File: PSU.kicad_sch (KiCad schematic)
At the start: 39 parts, among them Q401 2N7002, SW401 SW_Push, SW402 SW_Push, U3 TPPM0110DWPR, U402 AP7381-33SA-7, U403 AP63200WU

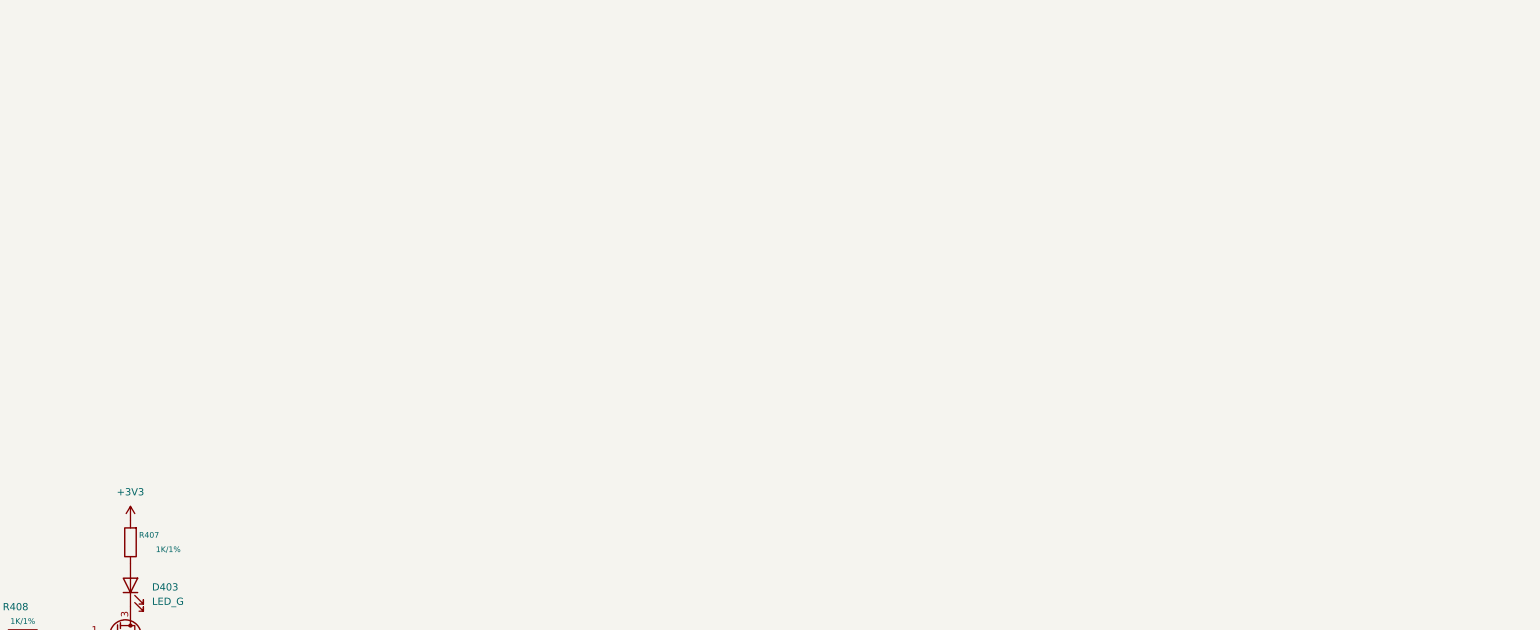
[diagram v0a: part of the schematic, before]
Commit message: some power stuff (unfinished)
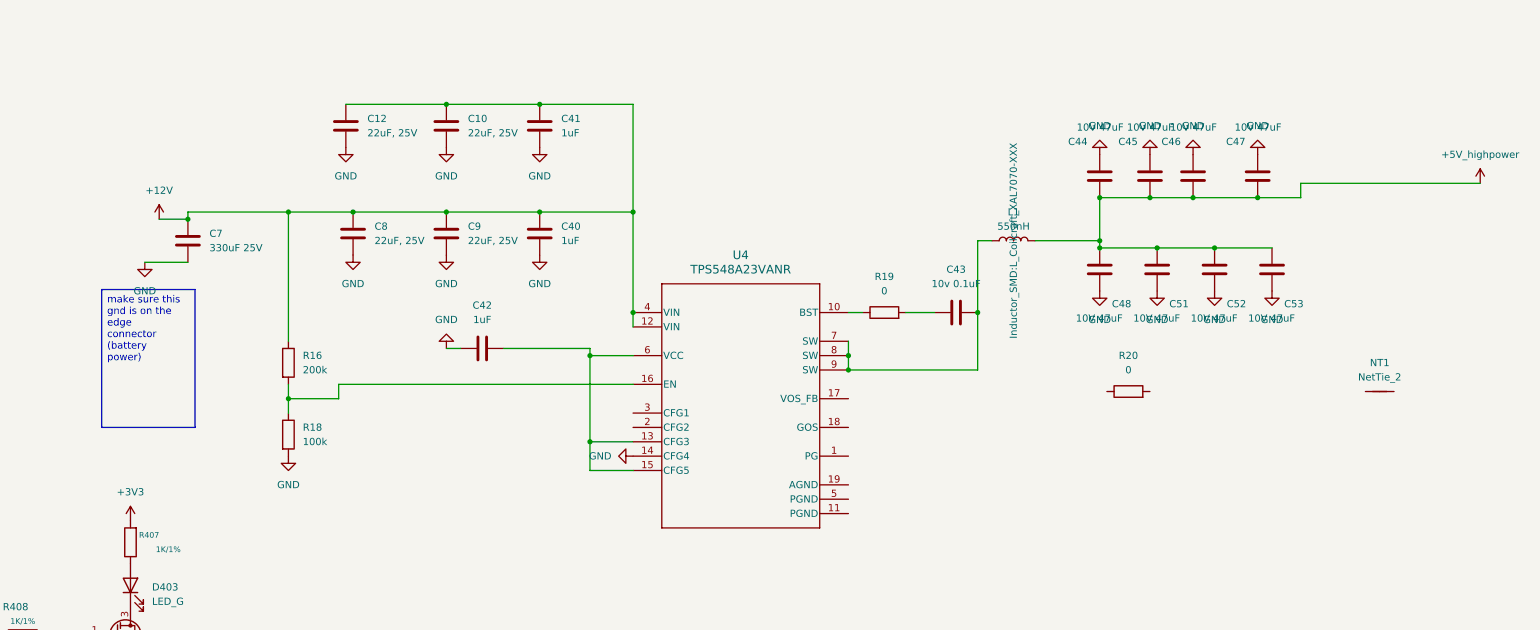
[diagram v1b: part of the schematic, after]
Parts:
- added C10, C12, C8, C9: 22uF, 25V, Capacitor_SMD:C_1206_3216Metric, symbol Device:C
- added C40, C41, C42: 1uF, A_DFRobot:C_0402_1005Metric, symbol Device:C
- added C43: 10v 0.1uF, A_DFRobot:C_0402_1005Metric, symbol Device:C
- added C44, C45, C46, C47, C48, C51, C52, C53: 10V 47uF, Capacitor_SMD:C_1210_3225Metric, symbol Device:C
- added C7: 330uF 25V, Capacitor_SMD:CP_Elec_8x11.9, symbol Device:C
- added L1: 550nH, Inductor_SMD:L_Coilcraft_XAL7070-XXX, symbol Device:L
- added NT1: NetTie_2, symbol Device:NetTie_2
- added R16: 200k, A_DFRobot:R_0402_1005Metric, symbol Device:R
- added R18: 100k, A_DFRobot:R_0402_1005Metric, symbol Device:R
- added R19, R20: 0, A_DFRobot:R_0402_1005Metric, symbol Device:R
- added U4: TPS548A23VANR, VAN0019A-MFG, symbol 2026-04-07_02-11-45:TPS548A23VANR
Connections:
- net +12V: now also C10.1, C12.1, C40.1, C41.1, C7.1, C8.1, C9.1, R16.1, U4.12 (VIN), U4.4 (VIN)
- net GND: now also C10.2, C12.2, C40.2, C41.2, C42.1, C44.1, C45.1, C46.1, C47.1, C48.1, C51.1, C52.1, C53.1, C7.2, C8.2, C9.2, R18.2, U4.14 (CFG4)
- new net: C43.1, R19.2
- new net: C43.2, L1.1, U4.7 (SW), U4.8 (SW), U4.9 (SW)
- new net: R19.1, U4.10 (BST)
- new net: R16.2, R18.1, U4.16 (EN)
- new net: C42.2, U4.13 (CFG3), U4.15 (CFG5), U4.6 (VCC)
- new net +5V_highpower: C44.2, C45.2, C46.2, C47.2, C48.2, C51.2, C52.2, C53.2, L1.2
